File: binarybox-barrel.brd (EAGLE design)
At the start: 142.2 x 91.4 mm, 29 parts, among them IC2 MAX7219CNG, X1 USBPTH

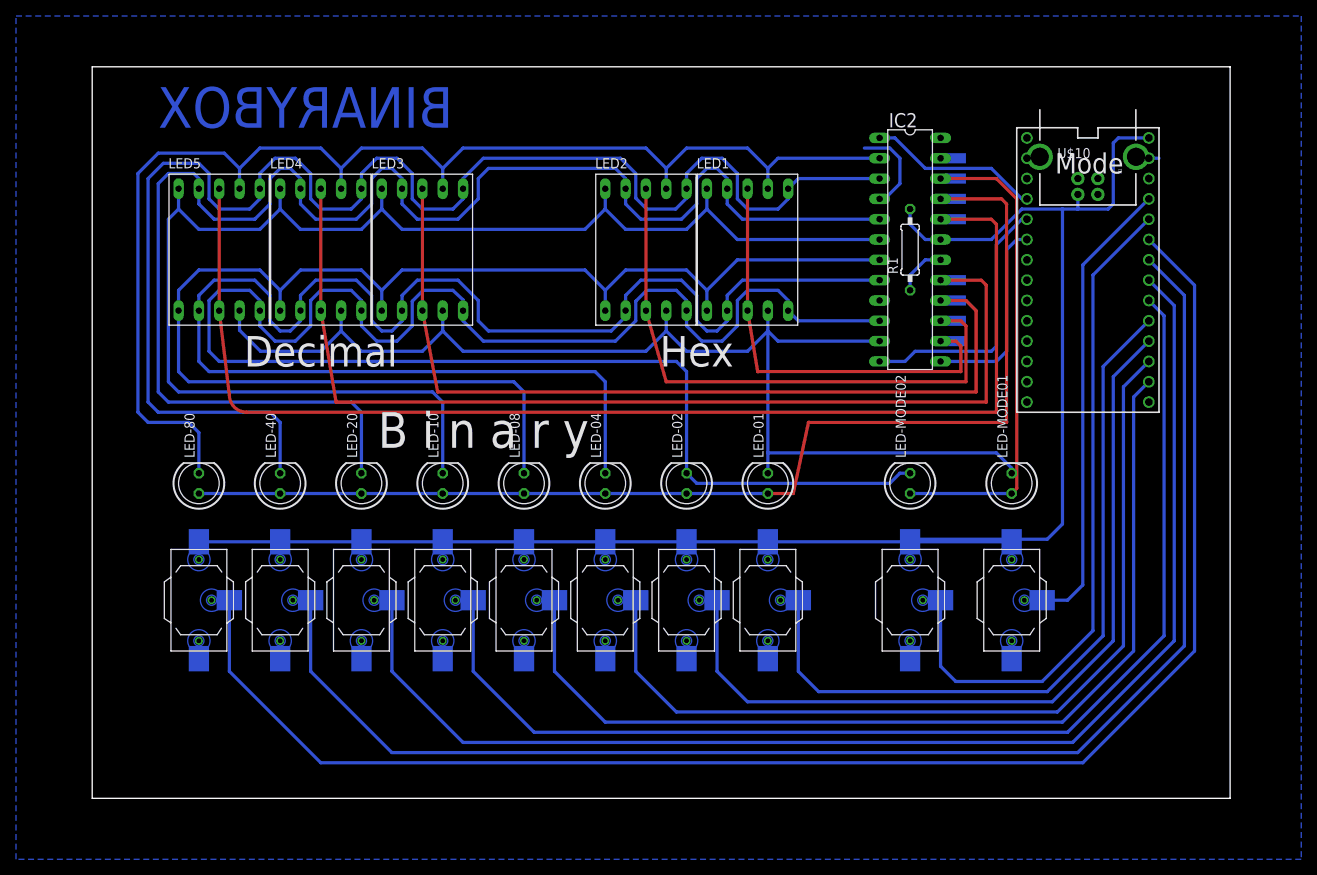
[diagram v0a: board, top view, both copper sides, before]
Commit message: cleaned up usb board and arduino sketch
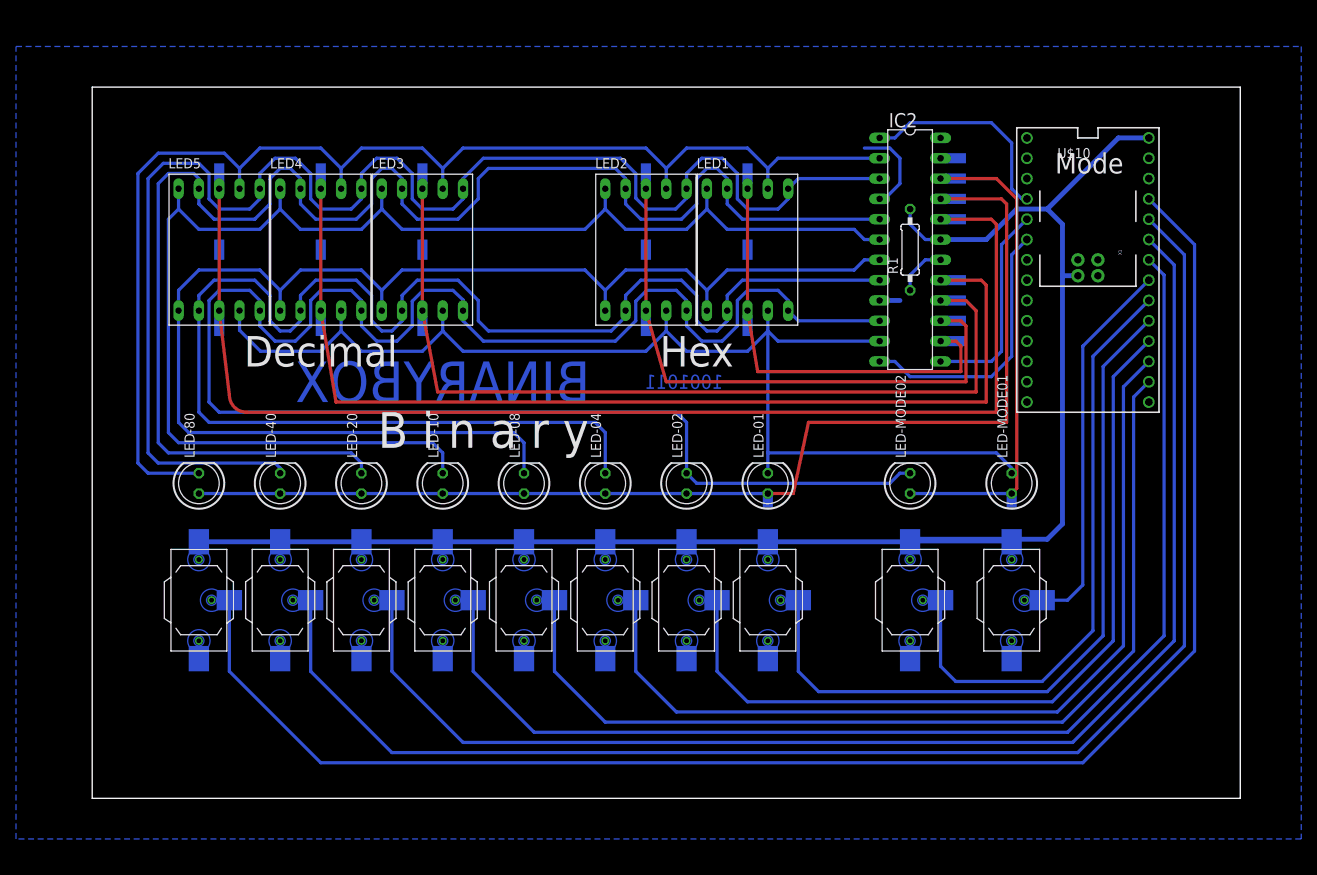
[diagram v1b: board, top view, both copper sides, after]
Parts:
- moved X1 10.2 mm to (124.5, 67.3)
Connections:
- net CLK: now also U$10.3; no longer U$10.4
- net INP10: now also U$10.20/A6; no longer U$10.18/A4
- net INP20: now also U$10.21/A7; no longer U$10.19/A5
- net INP40: now also U$10.22/A8; no longer U$10.20/A6
- net INP80: now also U$10.23/A9; no longer U$10.21/A7
- net LOAD: now also U$10.4; no longer U$10.3
- net MODE01: now also U$10.19/A5; no longer U$10.23/A9
- net MODE02: now also U$10.18/A4; no longer U$10.22/A8
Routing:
- net MODE02: track 85.1 -> 74.9 mm
- net MODE01: track 57.5 -> 47.4 mm
- net INP80: track 193.9 -> 198.9 mm
- net INP40: track 177.9 -> 183.0 mm
- net INP10: track 146.1 -> 151.2 mm
- net INP20: track 162.0 -> 167.1 mm
- net DIN: track 21.6 -> 26.5 mm
- net VCC: track 205.2 -> 201.7 mm
- net CLK: track 24.5 -> 26.0 mm
- net GND: track 12.7 -> 14.0 mm
- net SEGA: track 159.8 -> 160.5 mm
- net LOAD: track 33.2 -> 33.7 mm
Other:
- board size 142.2 x 91.4 mm -> 143.5 x 88.9 mm
- board text added: "1001011"
